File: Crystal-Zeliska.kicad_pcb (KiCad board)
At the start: 2 copper layers, 183.5 x 114.3 mm, 127 parts, among them K1 KEYSW, K10 KEYSW, K11 KEYSW, K12 KEYSW, K13 KEYSW, K14 KEYSW, K15 KEYSW, K16 KEYSW, K17 KEYSW, K18 KEYSW, K19 KEYSW, K2 KEYSW, K20 KEYSW, K21 KEYSW, K22 KEYSW, K23 KEYSW, K24 KEYSW, K25 KEYSW, K26 KEYSW, K27 KEYSW, K28 KEYSW, K29 KEYSW, K3 KEYSW, K30 KEYSW, K31 KEYSW, K4 KEYSW, K5 KEYSW, K6 KEYSW, K7 KEYSW, K8 KEYSW, K9 KEYSW, SW1 SW_Push_Open_Dual, U1 ProMicro, U2 TRRS

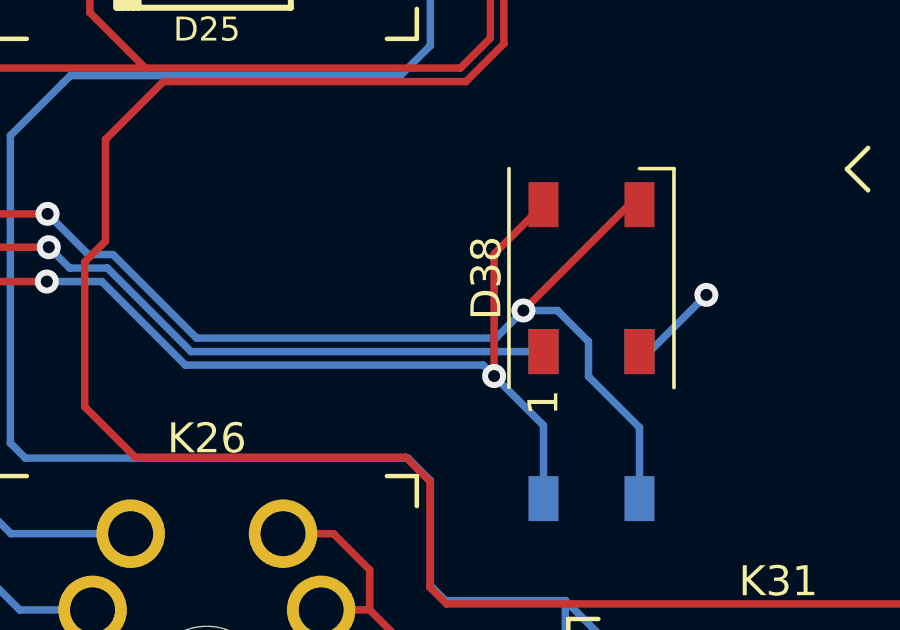
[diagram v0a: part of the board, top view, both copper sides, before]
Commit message: updated pcb
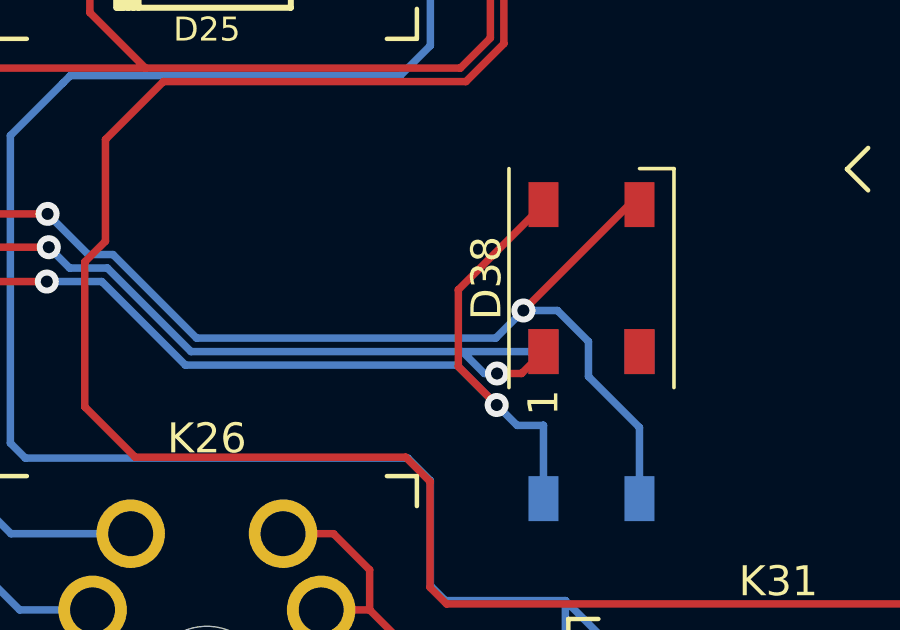
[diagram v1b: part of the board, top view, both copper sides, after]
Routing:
- net +5V: track 520.8 -> 524.5 mm, vias 14 -> 15
- net Net-(D38-Pad2): track 3.01 -> 0.34 mm, vias 1 -> 0
- net Net-(D38-Pad4): track 70.4 -> 72.4 mm
